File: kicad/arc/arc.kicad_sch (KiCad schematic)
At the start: 13 parts, among them J1 Conn_01x08, J2 Conn_01x03, J3 Conn_01x03, J4 Conn_01x03, J5 Conn_01x03, J6 Conn_01x03, J7 Conn_01x03, J8 Conn_01x03, J9 Conn_01x03, U1 ESP32-S3-WROOM-1U-N16R8, U2 BL5612, U3 TPS63020DSJR, U4 BL5612

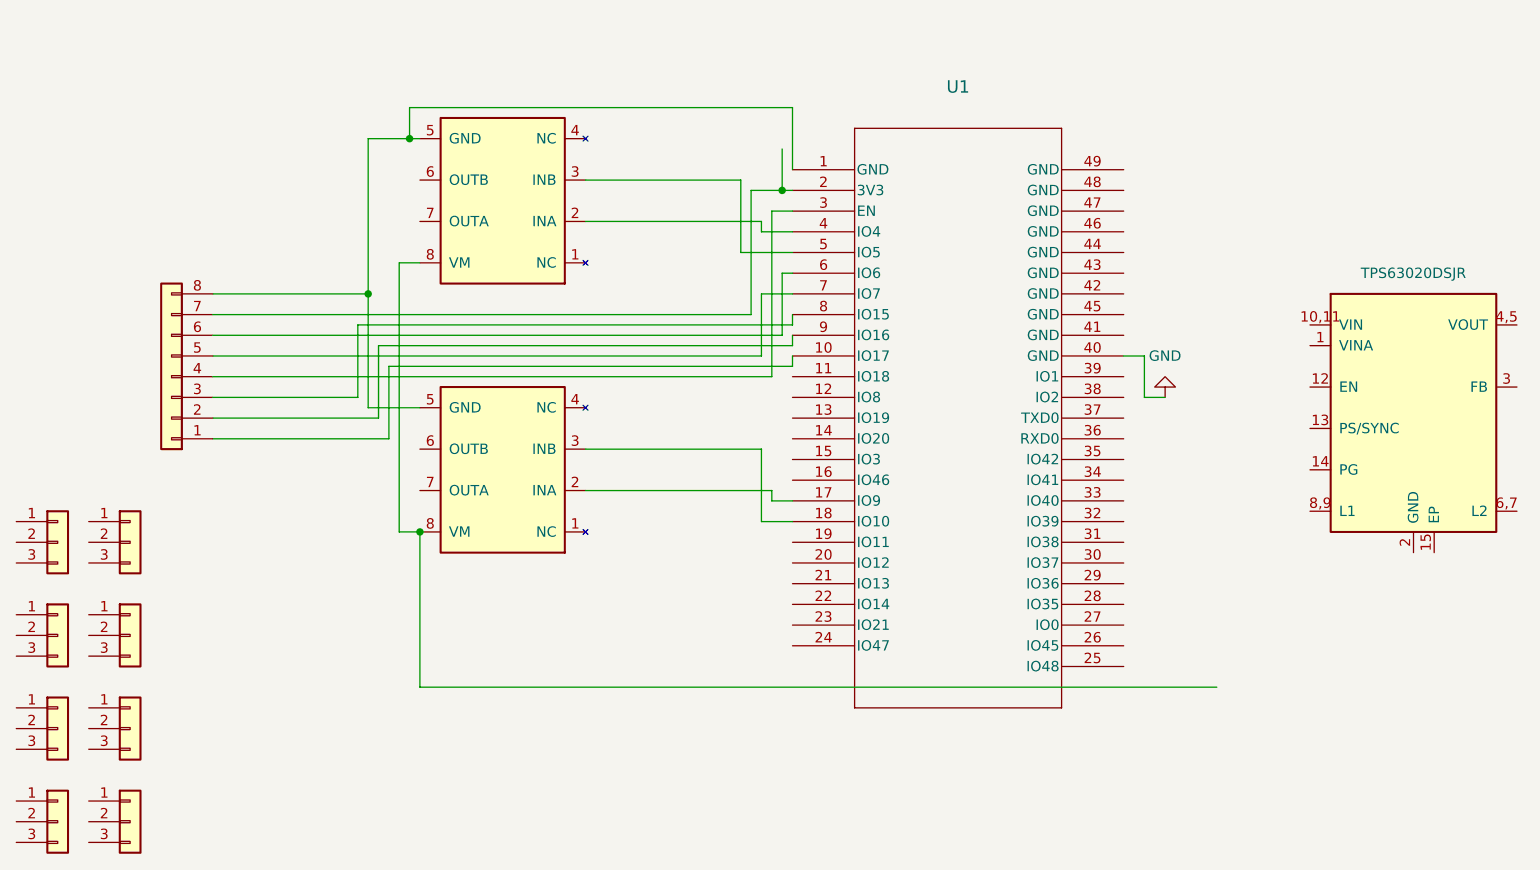
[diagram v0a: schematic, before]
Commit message: fixed it just a mare '#'
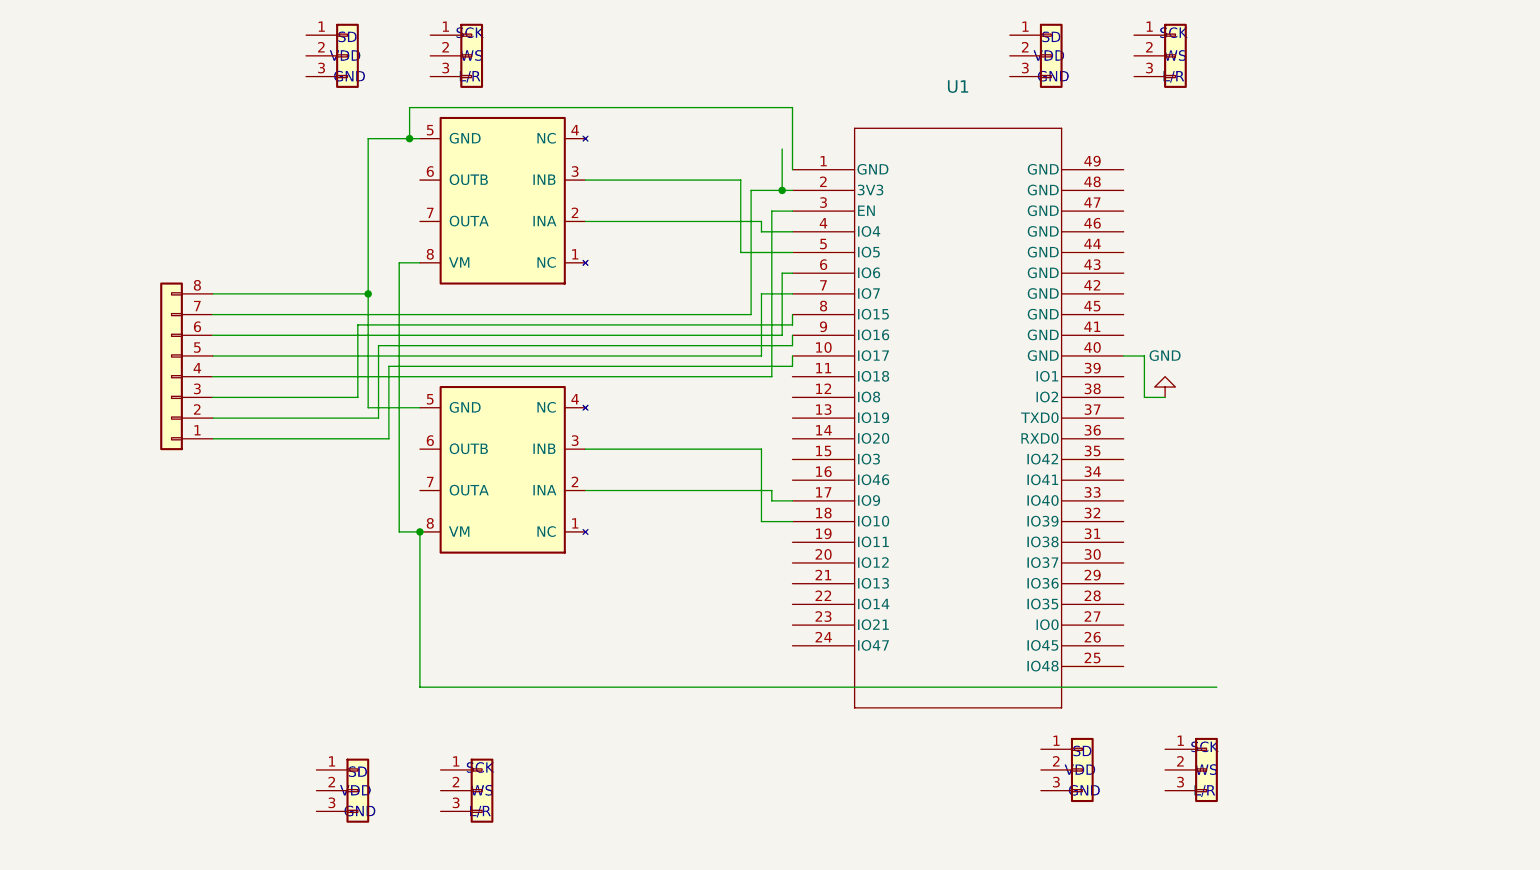
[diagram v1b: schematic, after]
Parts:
- removed U3: TPS63020DSJR, Package_SON:Texas_S-PVSON-N14_ThermalPad, symbol TPS63020DSJR:TPS63020DSJR
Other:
- note added: "GND"
- note added: "L/R"
- note added: "SCK"
- note added: "SD"
- note added: "VDD"
- note added: "WS"
